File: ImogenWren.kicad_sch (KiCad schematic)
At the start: 3 parts

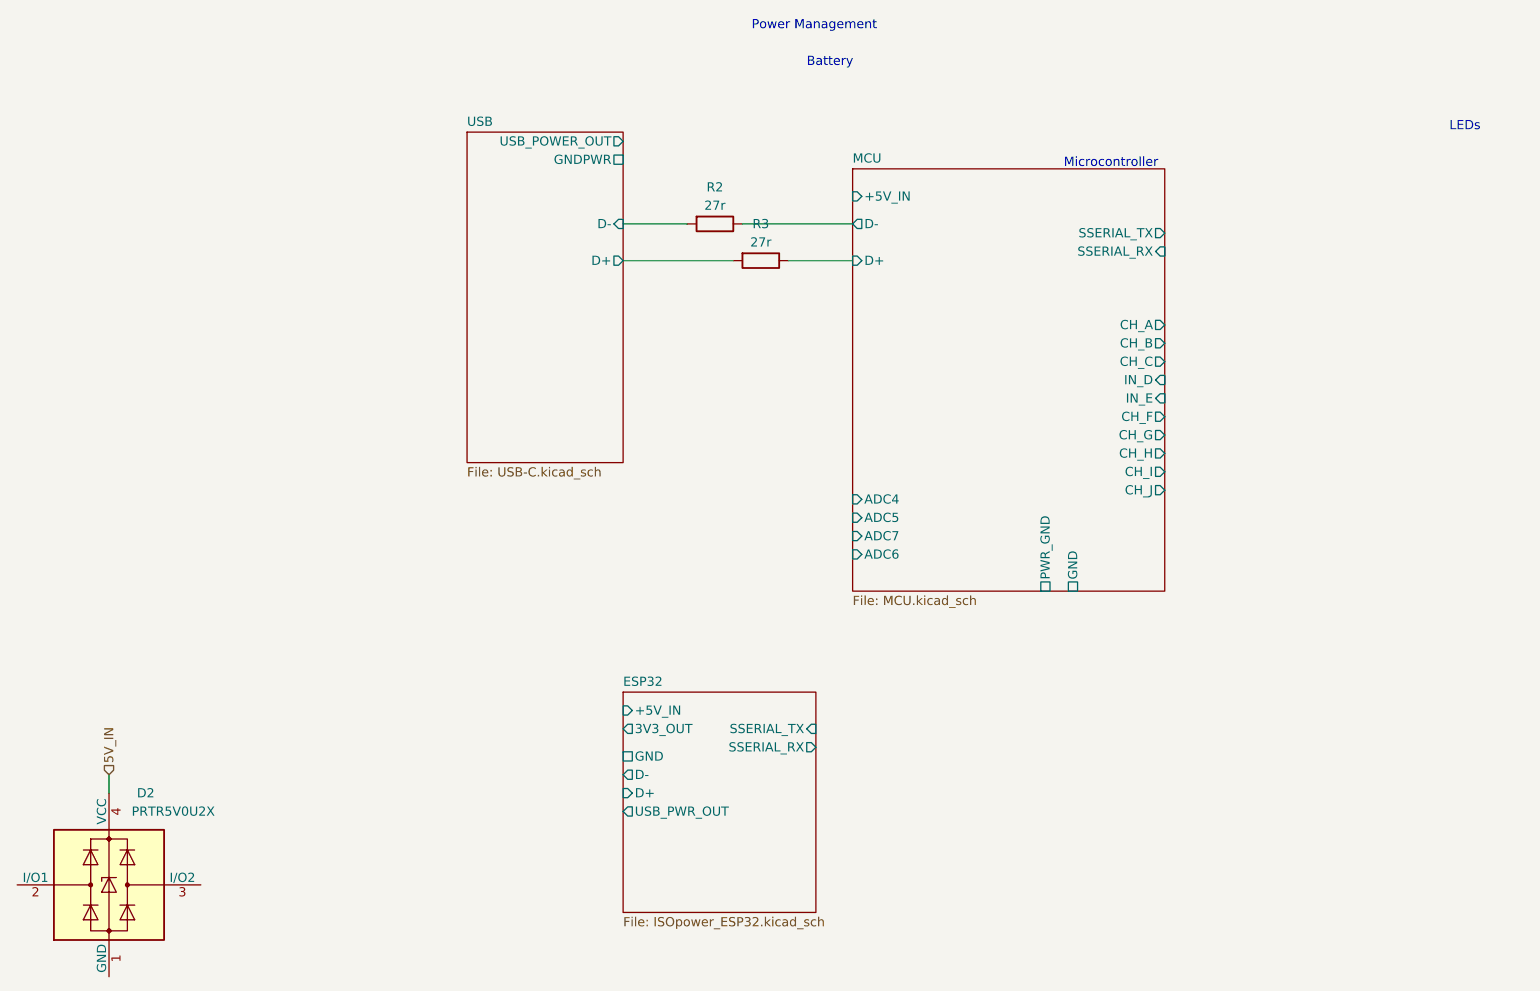
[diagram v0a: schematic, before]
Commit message: dfghdreg
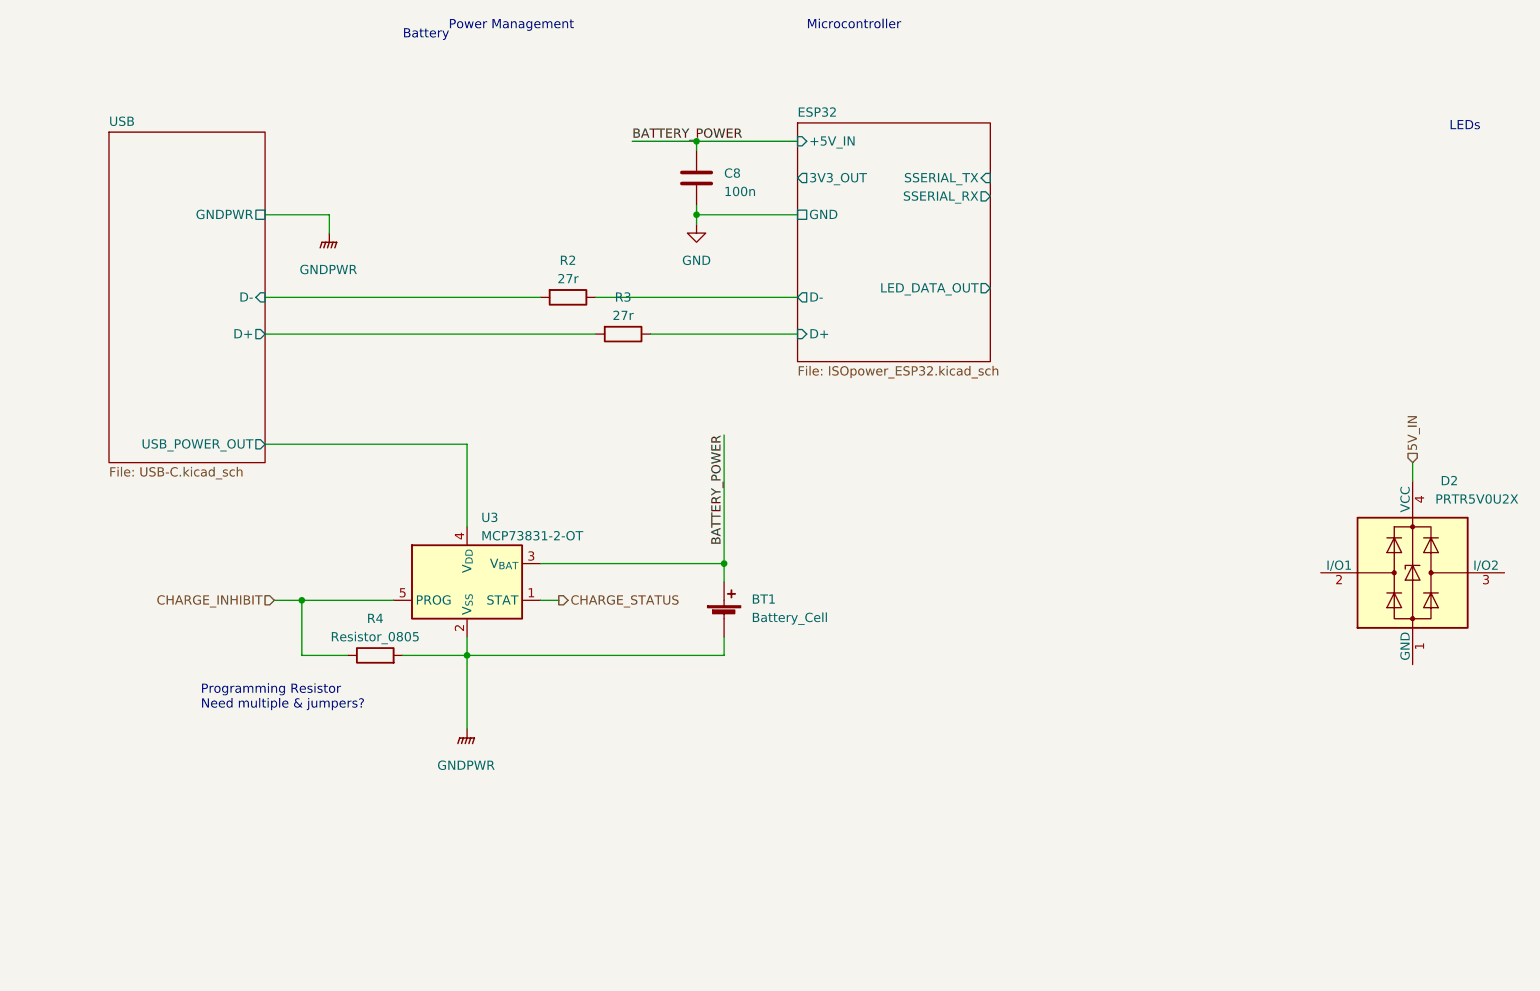
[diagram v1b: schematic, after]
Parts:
- added BT1: Battery_Cell, symbol Device:Battery_Cell
- added C8: 100n, Capacitor_SMD:C_0805_2012Metric_Pad1.18x1.45mm_HandSolder, symbol 000_Capacitor_Film_Immo:cap_film_0805
- added R4: Resistor_0805, Resistor_SMD:R_0805_2012Metric_Pad1.20x1.40mm_HandSolder, symbol 000_Resistors_Immo:Resistor_0805
- added U3: MCP73831-2-OT, Package_TO_SOT_SMD:SOT-23-5, symbol Battery_Management:MCP73831-2-OT
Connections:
- net MCU/D+ is gone; now on net ESP32/D+: R3.1
- net MCU/D- is gone; now on net ESP32/D-: R2.1
- net USB/USB_POWER_OUT: now also U3.4 (V_{DD})
- new net BATTERY_POWER: BT1.1 (+), C8.1, U3.3 (V_{BAT})
- new net CHARGE_INHIBIT: R4.1, U3.5 (PROG)
- new net CHARGE_STATUS: U3.1 (STAT)
- new net GND: C8.2
- new net GNDPWR: BT1.2 (-), R4.2, U3.2 (V_{SS})
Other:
- removed sheet MCU
- sheet ESP32 ports: added LED_DATA_OUT; removed USB_PWR_OUT
- note added: "Programming Resistor Need multiple & jumpers?"
- moved on the sheet: D2, R2, R3
